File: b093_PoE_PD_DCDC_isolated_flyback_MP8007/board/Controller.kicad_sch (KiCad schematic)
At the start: 19 parts, among them U1 MP8007, U2 CX9628-AL

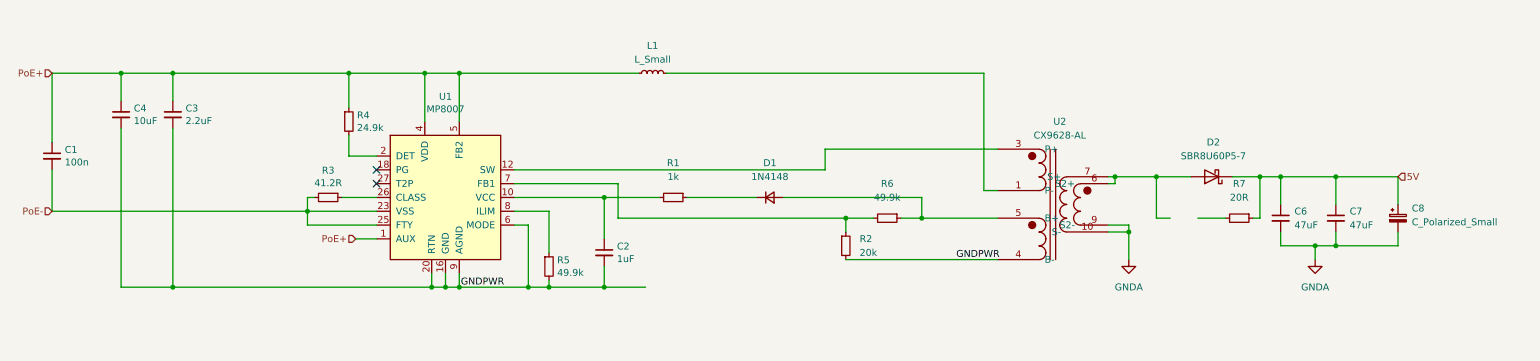
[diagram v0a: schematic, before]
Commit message: version 0.3
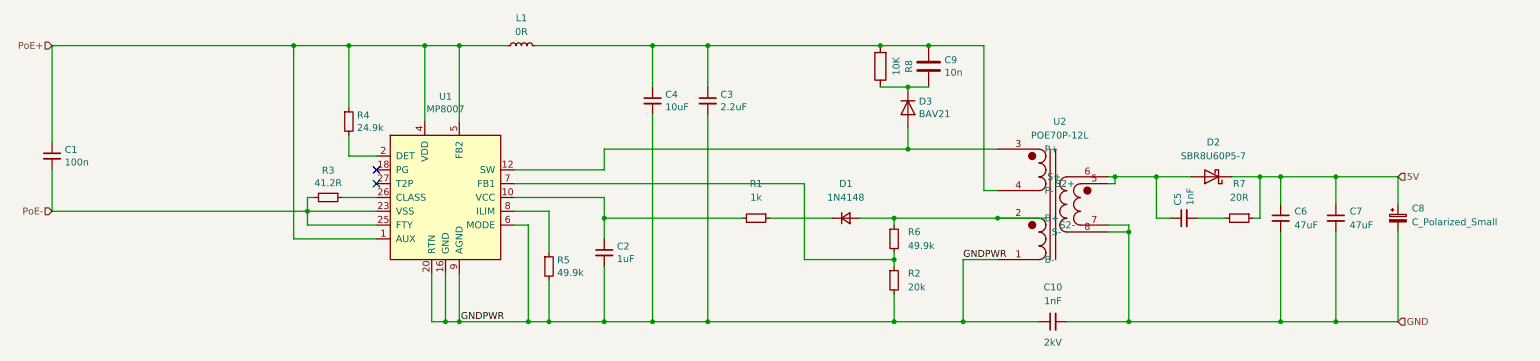
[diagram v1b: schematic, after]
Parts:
- added C10: 1nF, Capacitor_SMD:C_1825_4564Metric, symbol Device:C_Small
- added C5: 1nF, Capacitor_SMD:C_0603_1608Metric, symbol Device:C_Small
- added C9: 10n, Capacitor_SMD:C_0805_2012Metric, symbol Device:C
- added D3: BAV21, Diode_SMD:D_SOD-323_HandSoldering, symbol Device:D
- added R8: 10K, Resistor_SMD:R_1206_3216Metric, symbol Device:R
- L1: value L_Small -> 0R
- U2: value CX9628-AL -> POE70P-12L; footprint (none) -> local:Transformer_Coilcraft_POE70P; symbol local:CX9628-AL -> local:POE70P-50L
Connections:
- net GNDPWR: now also U2.1 (B-), C10.1; no longer U2.4 (B-)
- net PoE+: no longer C3.1, C4.1
- net at U1.12 (SW), U1.13, U2.3 (P+): now also D3.2 (A)
- net at R7.2: now also C5.2
- net at L1.2: now also C3.1, C4.1, U2.4 (P-), C9.1, R8.2; no longer U2.1 (P-)
- net at D1.2 (A), R6.1: now also U2.2 (B+); no longer U2.5 (B+)
- net at D2.2 (A), U2.6 (S+): now also U2.5 (S2+), C5.1; no longer U2.7 (S+)
- net GNDA renamed GND
- net GND: now also U2.7 (S2-), U2.8 (S-), C10.2; no longer U2.10 (S-), U2.9 (S2-)
- new net: C9.2, D3.1 (K), R8.1
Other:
- moved on the sheet: C3, C4, D1, L1, R1, R2, R6
